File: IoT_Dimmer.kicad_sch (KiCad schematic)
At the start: 0 parts

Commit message: add lib
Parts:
- added C1: 0.05uF, symbol Device:C
- added C2: 0.01uF, symbol Device:C
- added D1: BTA204S-800, symbol Triac_Thyristor:Generic_Triac_A1A2G
- added J1, J2: Screw_Terminal_01x02, symbol Connector:Screw_Terminal_01x02
- added PS1: IRM-02-3.3, Converter_ACDC:Converter_ACDC_MeanWell_IRM-02-xx_THT, symbol Converter_ACDC:IRM-02-3.3
- added R1: 360, symbol Device:R
- added R2: 470, symbol Device:R
- added R3: 39, symbol Device:R
- added U1: MOC3021M, symbol Relay_SolidState:MOC3021M
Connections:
- new net: R1.1, U1.6
- new net: C1.1, R1.2, R2.1
- new net: D1.2 (A2), R2.2, R3.1
- new net: C2.1, R3.2
- new net: C1.2, C2.2, D1.1 (A1)
- new net: D1.3 (G), U1.4
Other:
- company: (none) -> No
- title: (none) -> IoT Dimmer

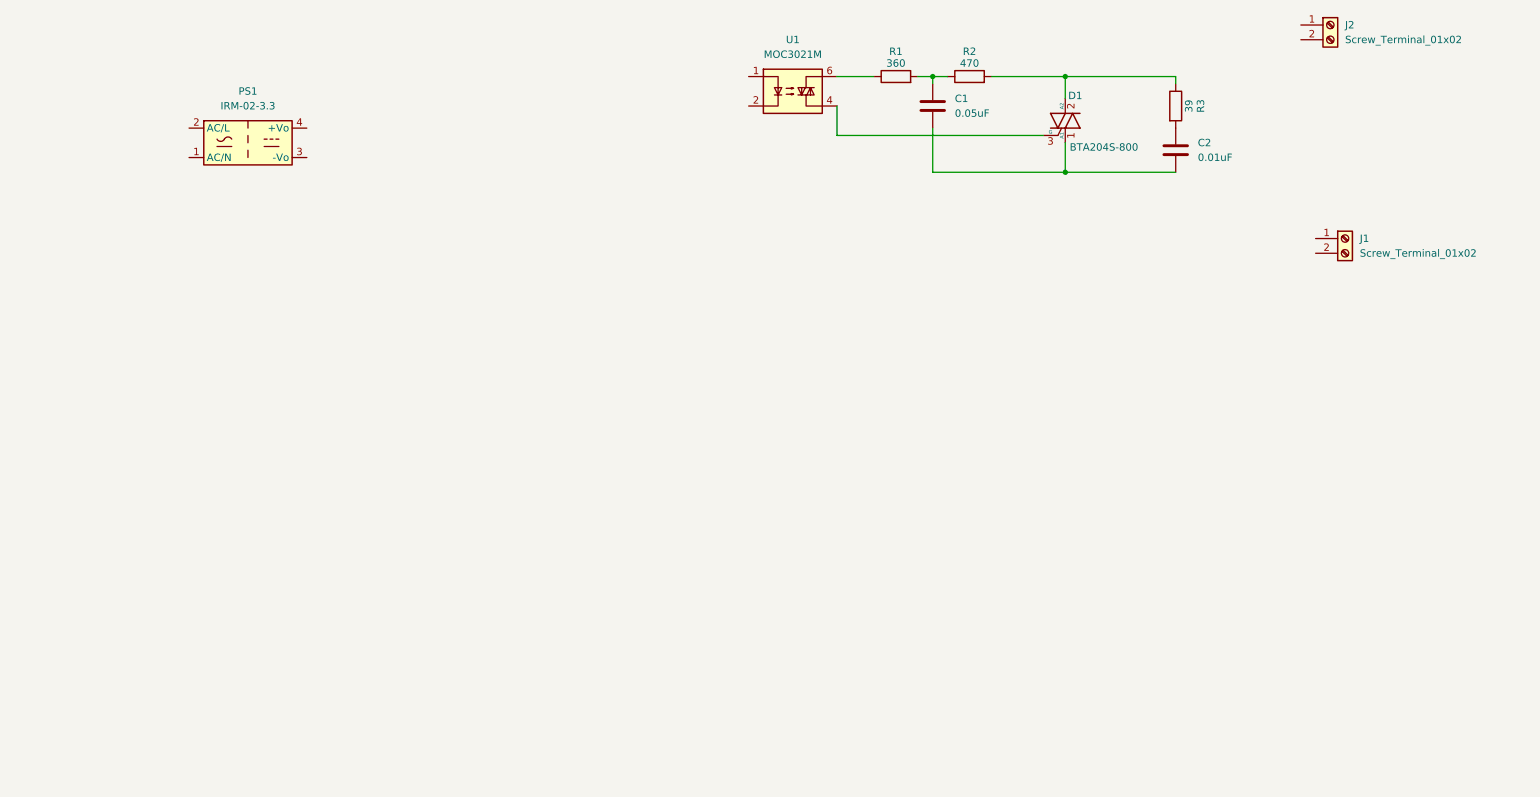
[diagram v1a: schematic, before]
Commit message: CPU and 220
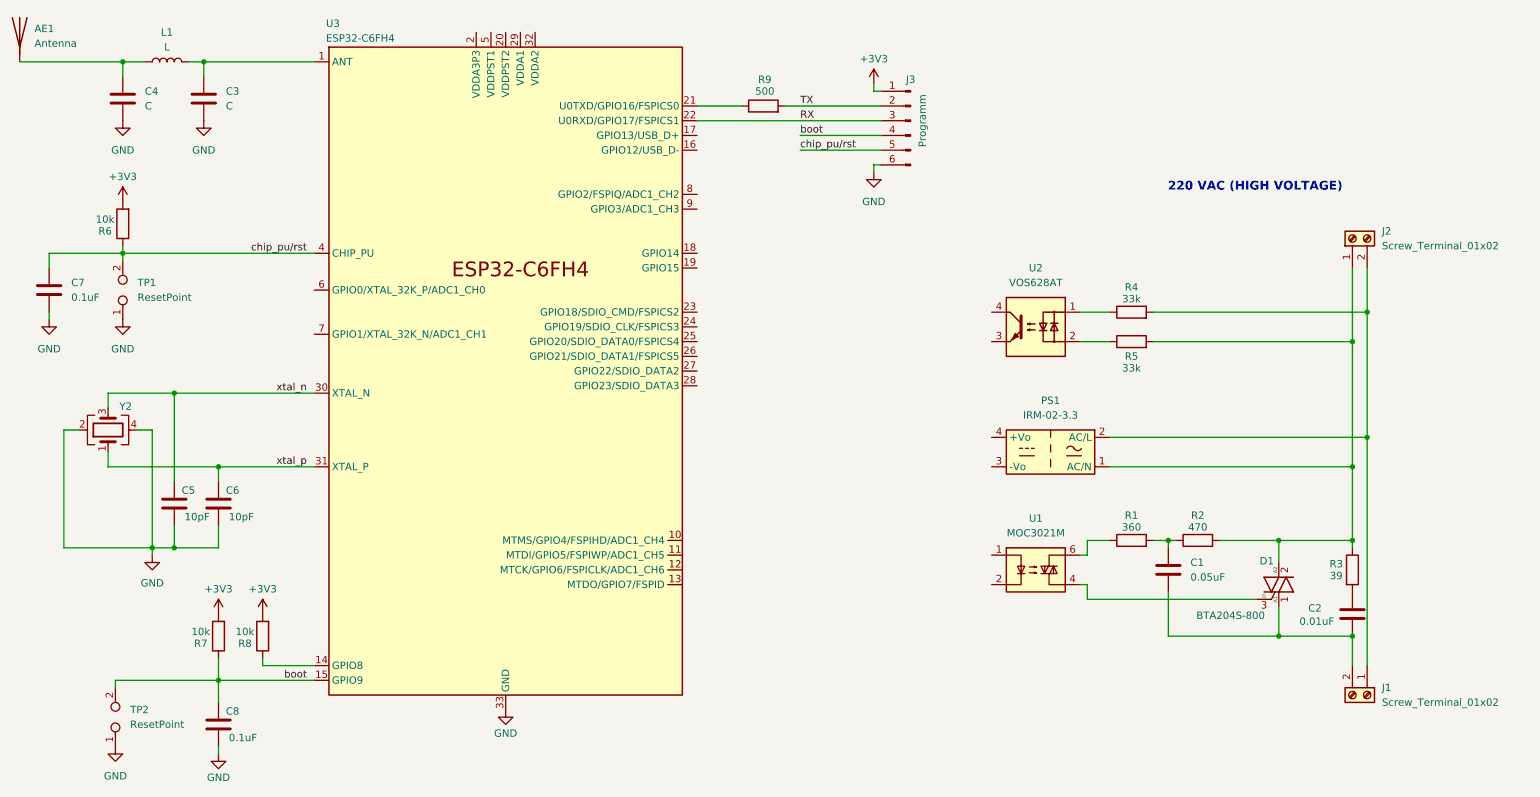
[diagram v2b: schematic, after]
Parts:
- added AE1: Antenna, symbol Device:Antenna
- added C3, C4: C, symbol Device:C
- added C5, C6: 10pF, symbol Device:C
- added C7, C8: 0.1uF, symbol Device:C
- added J3: Conn_01x06_Pin, symbol Connector:Conn_01x06_Pin
- added L1: L, symbol Device:L
- added R4, R5: 33k, symbol Device:R
- added R6, R7, R8: 10k, symbol Device:R
- added R9: 500, symbol Device:R
- added TP1, TP2: ResetPoint, symbol Connector:TestPoint_2Pole
- added U2: VOS628AT, VOS628AT:SOIC127P700X210-4N, symbol VOS628AT:VOS628AT
- added U3: ESP32-C6FH4, Package_DFN_QFN:QFN-32-1EP_5x5mm_P0.5mm_EP3.6x3.6mm, symbol PCM_Espressif:ESP32-C6FH4
- added Y2: Crystal_GND24, symbol Device:Crystal_GND24
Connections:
- net at PS1.1 (AC/N): now also D1.2 (A2), J2.1 (Pin_1), R2.2, R3.1, R5.2
- net at PS1.2 (AC/L): now also J1.1 (Pin_1), J2.2 (Pin_2), R4.2
- net at C1.2, C2.2, D1.1 (A1): now also J1.2 (Pin_2)
- new net: R9.1, U3.21 (U0TXD/GPIO16/FSPICS0)
- new net: R4.1, U2.1
- new net: R5.1, U2.2
- new net: R8.1, U3.14 (GPIO8)
- new net: AE1.1 (A), C4.1, L1.1
- new net: C3.1, L1.2, U3.1 (ANT)
- new net: U3.2 (VDDA3P3), U3.3 (VDDA3P3)
- new net +3V3: J3.1 (Pin_1), R6.2, R7.2, R8.2
- new net GND: C3.2, C4.2, C5.2, C6.2, C7.2, C8.2, J3.6 (Pin_6), TP1.1, TP2.1, U3.33 (GND), Y2.2, Y2.4
- new net RX: J3.3 (Pin_3), U3.22 (U0RXD/GPIO17/FSPICS1)
- new net TX: J3.2 (Pin_2), R9.2
- new net boot: C8.1, J3.4 (Pin_4), R7.1, TP2.2, U3.15 (GPIO9)
- new net chip_pu/rst: C7.1, J3.5 (Pin_5), R6.1, TP1.2, U3.4 (CHIP_PU)
- new net xtal_n: C5.1, U3.30 (XTAL_N), Y2.3
- new net xtal_p: C6.1, U3.31 (XTAL_P), Y2.1
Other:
- note added: "220 VAC (HIGH VOLTAGE)"
- moved on the sheet: C1, C2, D1, J1, J2, PS1, R1, R2, R3, U1
